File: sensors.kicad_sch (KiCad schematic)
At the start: 13 parts, among them U3 BMP581, U4 BNO085, Y2 Crystal

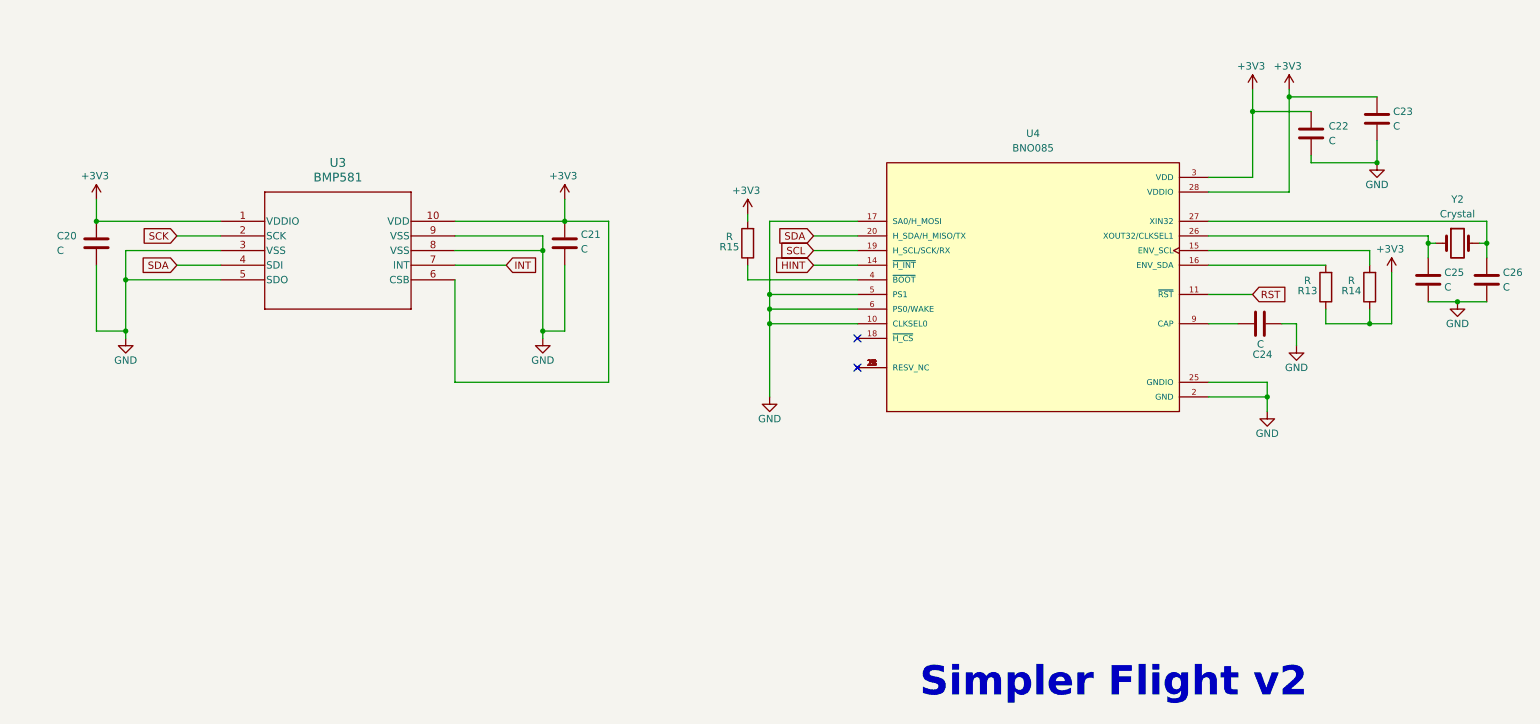
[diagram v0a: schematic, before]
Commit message: addecd stuff
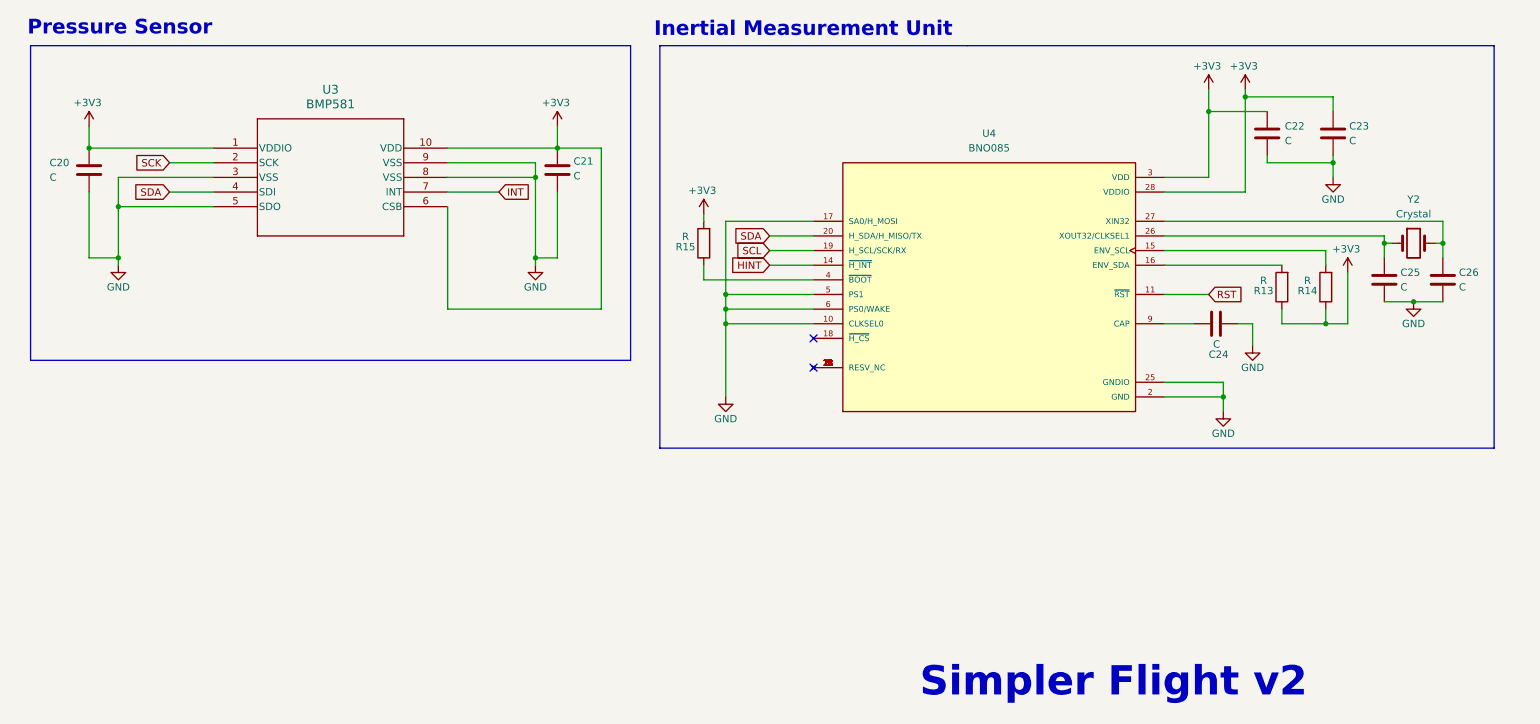
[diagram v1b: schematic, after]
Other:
- note added: "Inertial Measurement Unit"
- note added: "Pressure Sensor"
- moved on the sheet: C20, C21, C22, C23, C24, C25, C26, R13, R14, R15, U3, U4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

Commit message: Initiliase main components
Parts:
- C20, C21, C22, C23, C24, C25, C26: footprint (none) -> Capacitor_SMD:C_0805_2012Metric
- R13, R14, R15: footprint (none) -> Resistor_SMD:R_0805_2012Metric_Pad1.20x1.40mm_HandSolder
- U3: footprint footprints:QFN10_BMP581_BOS -> BMP581:QFN10_BMP581_BOS
- Y2: footprint (none) -> Crystal:Crystal_SMD_0603-2Pin_6.0x3.5mm_HandSoldering
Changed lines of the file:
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@@
 			)
 		)
-		(property "Footprint" "footprints:QFN10_BMP581_BOS"
+		(property "Footprint" "BMP581:QFN10_BMP581_BOS"
 			(at 55.88 81.28 0)
 			(effects
@@
 			)
 		)
-		(property "Footprint" ""
+		(property "Footprint" "Capacitor_SMD:C_0805_2012Metric"
 			(at 251.1552 82.55 0)
 			(effects
@@
 			)
 		)
-		(property "Footprint" ""
+		(property "Footprint" "Capacitor_SMD:C_0805_2012Metric"
 			(at 260.0452 107.95 0)
 			(effects
@@
 			)
 		)
-		(property "Footprint" ""
+		(property "Footprint" "Capacitor_SMD:C_0805_2012Metric"
 			(at 239.7252 82.55 0)
 			(effects
@@
 			)
 		)
-		(property "Footprint" ""
+		(property "Footprint" "Resistor_SMD:R_0805_2012Metric_Pad1.20x1.40mm_HandSolder"
 			(at 243.078 105.41 90)
 			(effects
@@
 			)
 		)
-		(property "Footprint" ""
+		(property "Footprint" "Crystal:Crystal_SMD_0603-2Pin_6.0x3.5mm_HandSoldering"
 			(at 264.16 97.79 0)
 			(effects
@@
 			)
 		)
-		(property "Footprint" ""
+		(property "Footprint" "Resistor_SMD:R_0805_2012Metric_Pad1.20x1.40mm_HandSolder"
 			(at 250.698 105.41 90)
 			(effects
@@
 			)
 		)
-		(property "Footprint" ""
+		(property "Footprint" "Capacitor_SMD:C_0805_2012Metric"
 			(at 116.5352 88.9 0)
 			(effects
@@
 			)
 		)
-		(property "Footprint" ""
+		(property "Footprint" "Capacitor_SMD:C_0805_2012Metric"
 			(at 35.2552 88.9 0)
 			(effects
@@
 			)
 		)
-		(property "Footprint" ""
+		(property "Footprint" "Capacitor_SMD:C_0805_2012Metric"
 			(at 270.2052 107.95 0)
 			(effects
@@
 			)
 		)
-		(property "Footprint" ""
+		(property "Footprint" "Capacitor_SMD:C_0805_2012Metric"
 			(at 226.06 112.7252 0)
 			(effects
@@
 			)
 		)
-		(property "Footprint" ""
+		(property "Footprint" "Resistor_SMD:R_0805_2012Metric_Pad1.20x1.40mm_HandSolder"
 			(at 142.748 97.79 90)
 			(effects
